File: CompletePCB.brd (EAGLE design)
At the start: 113 x 70.8 mm, 86 parts, among them IC1 SA602AD_01,118, IC3 L78L08ABUTR, IC4 LM386M-1, T1 2N3565, T2 2N3565, T3 2N3565, T4 2N3565, T5 2N3565, X1 1-227161-0

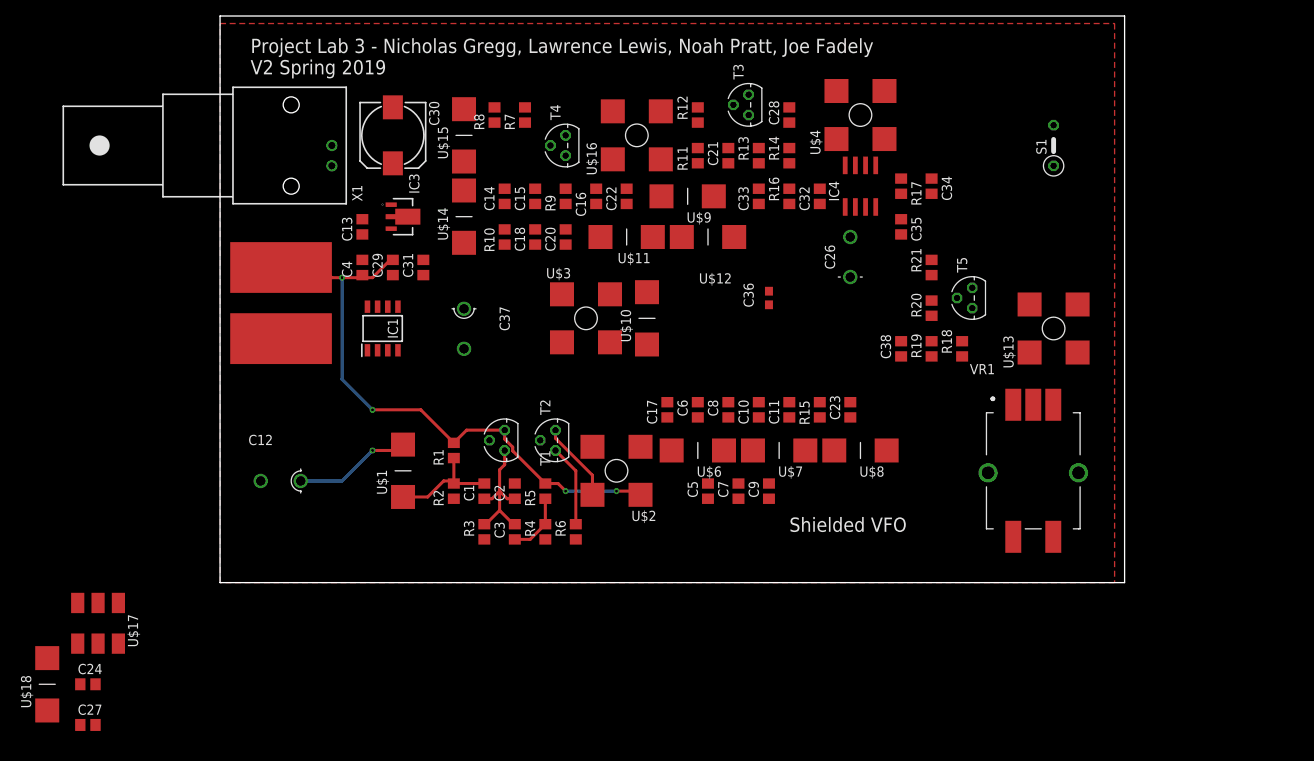
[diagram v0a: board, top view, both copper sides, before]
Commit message: Changes Made over time
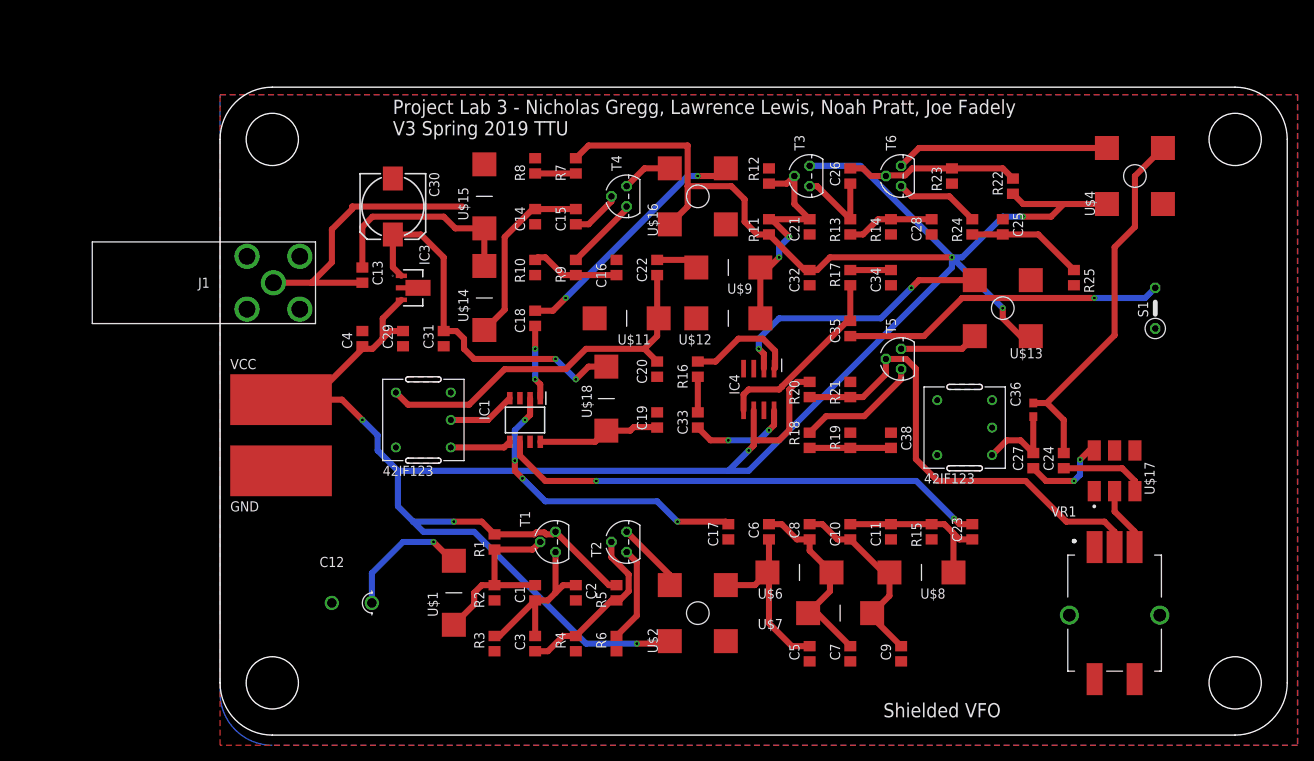
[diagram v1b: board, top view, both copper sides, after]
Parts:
- removed C37: GKG20015, SamacSys_Parts:GKG20015
- removed X1: 1-227161-0, con-coax:AMP_227161
- added C19, C25: (no value), eagle-ltspice:C0805
- added J1: 5413631-1, SamacSys_Parts:54136311
- added R22, R23, R24, R25: (no value), resistor:R0805
- added T6: 2N3565, transistor:TO92
- C26: value GKG20015 -> (none); device SamacSys_Parts:GKG20015 -> eagle-ltspice:C0805
- U$10: value WOUNDINDUCTOR -> 42IF123; device Custom:WOUNDINDUCTOR -> Custom:42IF123
- U$3: value RFTRANSFORMER -> 42IF123; device Custom:RFTRABSFORMER -> Custom:42IF123
- moved U$17 128.4 mm to (111.8, 33.0)
- moved C24 125.1 mm to (105.4, 34.3), turned to 90 degrees
- moved C27 122.6 mm to (101.6, 34.3), turned to 90 degrees
- moved U$18 78.4 mm to (48.3, 42.0), turned to 180 degrees
- moved U$10 42.0 mm to (93.0, 38.4), turned to 180 degrees
- moved C36 35.9 mm to (101.6, 40.6)
- moved U$4 35.1 mm to (114.3, 69.8)
- moved C33 29.0 mm to (59.7, 39.4)
- moved IC4 28.4 mm to (67.3, 43.2), turned to 180 degrees
- moved C9 26.2 mm to (85.1, 10.2)
- moved C7 24.7 mm to (78.7, 10.2)
- moved R16 24.4 mm to (59.7, 45.7), turned to 270 degrees
- moved U$3 24.0 mm to (25.4, 39.4), turned to 180 degrees
- moved C5 24.0 mm to (73.7, 10.2)
- moved S1 24.0 mm to (116.8, 53.3)
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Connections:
- new net N$2: C30.+, C31.2, IC3.1, U$18.2
- new net N$34: C19.1, IC1.8, U$18.1
- new net N$37: R24.2, T6.3
- new net N$38: C25.1, R24.1, R25.2
- new net N$43: C13.2, U$14.1, U$15.2
- net GND: now also C19.2, C25.2, J1.2, J1.3, J1.4, J1.5, R23.1, R25.1, U$10.P$1, U$3.P$4; no longer C13.2, C26.1, U$10.1, U$18.1, U$3.P$1, X1.2
- net IF: now also U$3.P$5; no longer U$3.P$2
- net N$15: now also J1.1; no longer U$14.1, U$15.2, X1.1
- net N$20: now also U$3.P$2; no longer C37.2, U$3.P$4
- net N$21: now also U$3.P$1; no longer C37.1, U$3.P$3
- net N$26: now also T6.1; no longer T3.1
- net N$27: now also U$10.P$2; no longer C26.2, U$10.2
- net N$39: now also C26.1, R13.2, T3.3; no longer C30.+, C31.2, IC1.8, IC3.1, U$18.2
- net N$6: now also C26.2, R22.1, R23.2, T6.2; no longer R13.2, T3.3
- net VCC: now also R22.2, T3.1
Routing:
- net VCC: track 73.0 -> 355.5 mm, vias 4 -> 7
- net VFO: track 0.00 -> 61.8 mm, vias 0 -> 2
- net N$28: track 0.00 -> 58.7 mm
- net QD: track 0.00 -> 47.7 mm
- net IF: track 0.00 -> 47.0 mm
- net N$2: track 0.00 -> 46.6 mm, vias 0 -> 2
- net N$46: track 0.00 -> 40.6 mm, vias 0 -> 1
- net N$23: track 0.00 -> 39.3 mm, vias 0 -> 4
- net N$15: track 0.00 -> 36.5 mm
- net N$35: track 0.00 -> 34.0 mm, vias 0 -> 2
- net RF: track 0.00 -> 31.2 mm, vias 0 -> 2
- net N$31: track 0.00 -> 30.6 mm, vias 0 -> 2
- net N$26: track 0.00 -> 26.6 mm
- net N$43: track 0.00 -> 25.1 mm
- net N$10: track 0.00 -> 24.3 mm
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- added copper zone on layer 16, net GND
- added copper zone on layer 1, net HOLE
- added copper zone on layer 1, net HOLE1
- added copper zone on layer 1, net HOLE2
- added copper zone on layer 1, net HOLE3
- added copper zone on layer 16, net PORT
- added copper zone on layer 16, net PORT1
- added copper zone on layer 16, net PORT2
- added copper zone on layer 16, net PORT3
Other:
- board size 113 x 70.8 mm -> 133.3 x 81 mm
- board text added: "Project Lab 3 - Nicholas Gregg, Lawrence Lewis, Noah Pratt, Joe Fadely V3 Spring 2019 TTU"
- board text removed: "Project Lab 3 - Nicholas Gregg, Lawrence Lewis, Noah Pratt, Joe Fadely V2 Spring 2019"
